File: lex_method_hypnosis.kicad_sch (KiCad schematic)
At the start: 4 parts

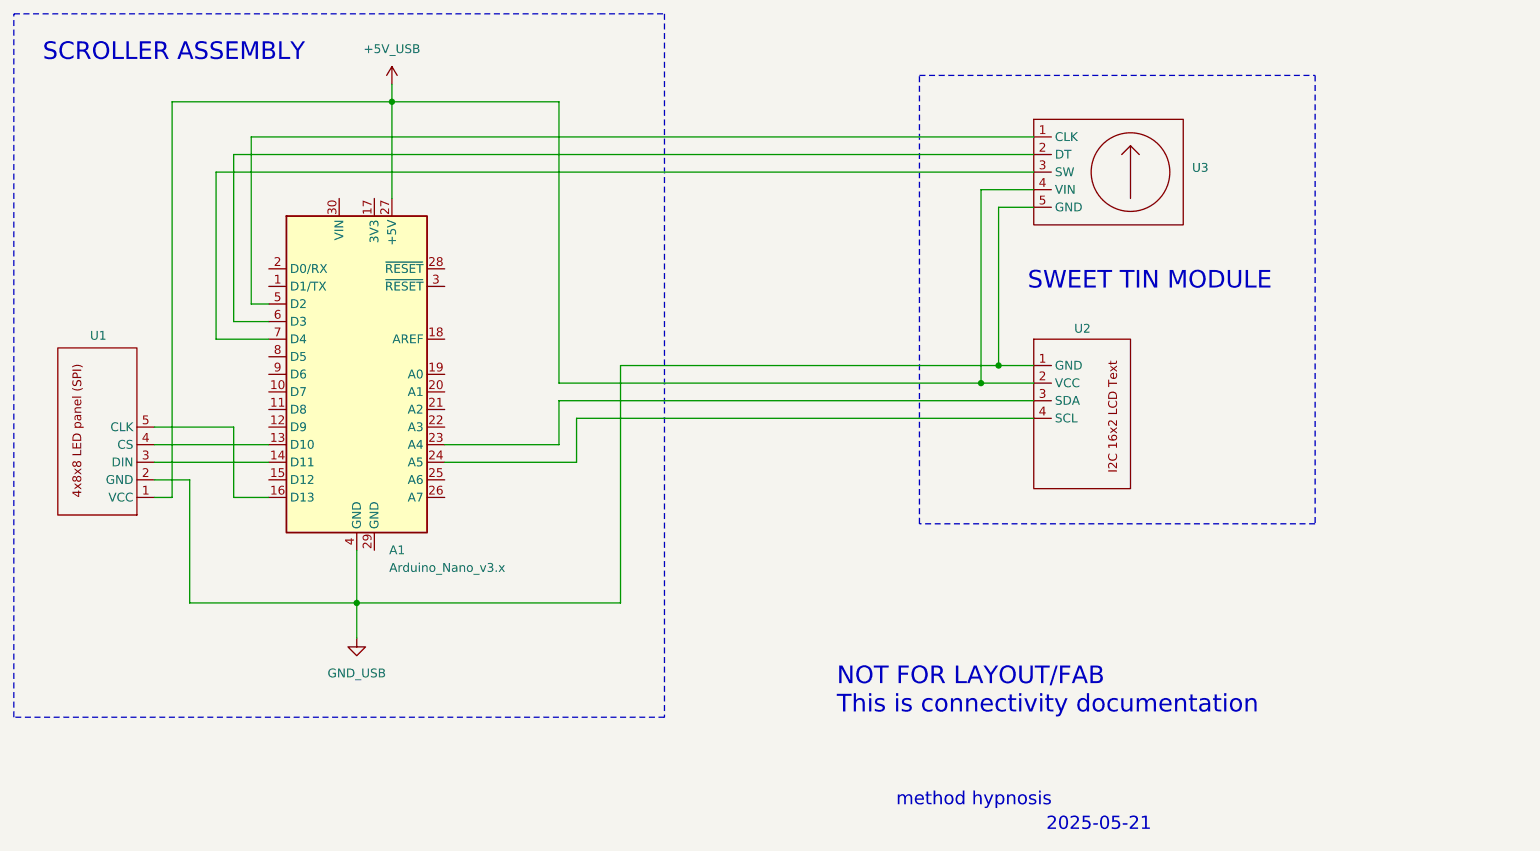
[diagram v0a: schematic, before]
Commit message: About to wire up connectors (gulpoid)
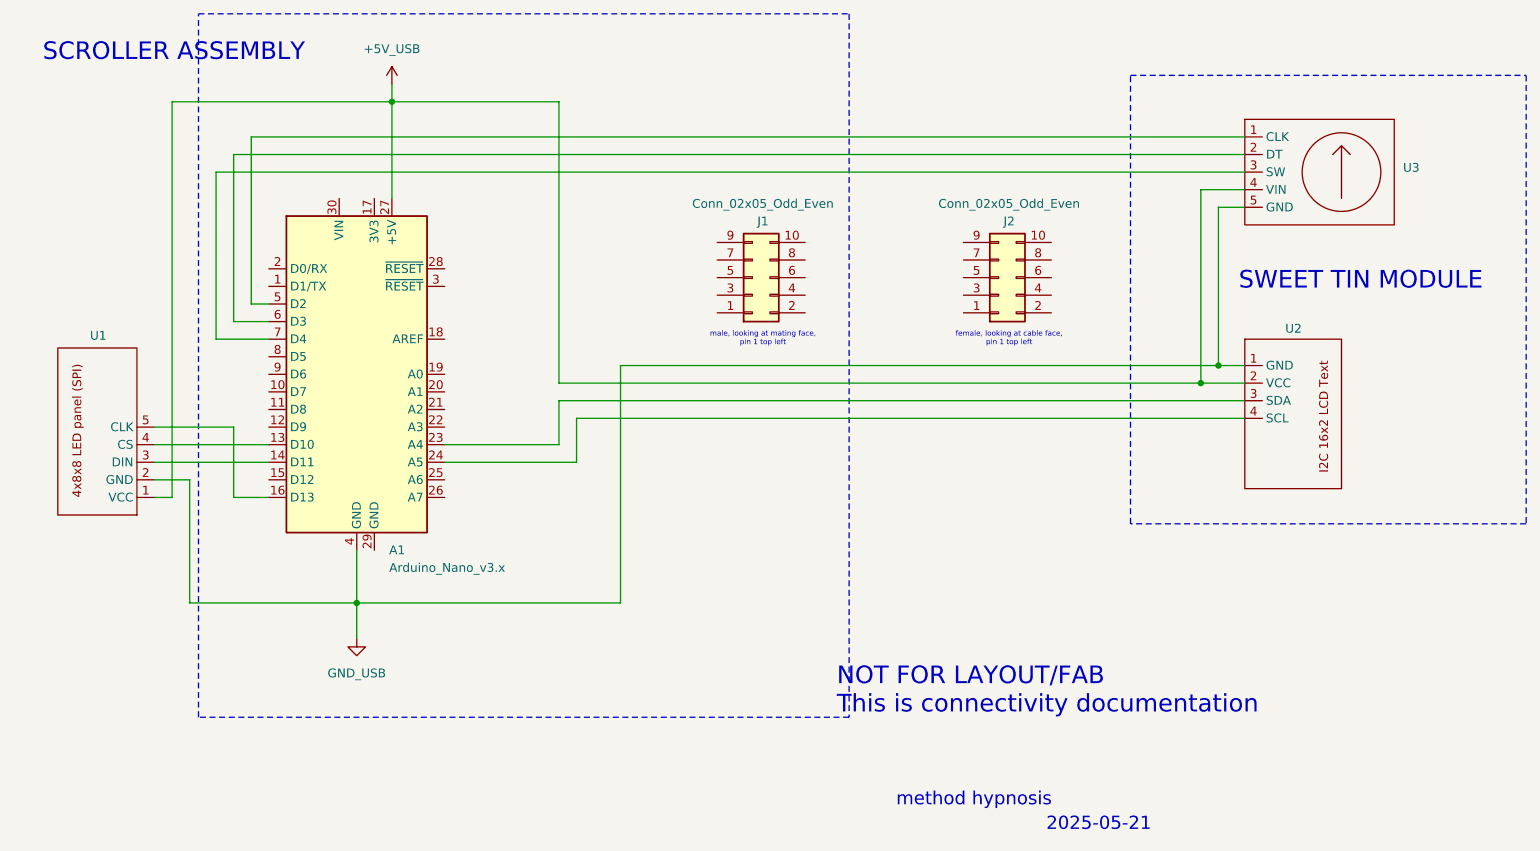
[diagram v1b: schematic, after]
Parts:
- added J1, J2: Conn_02x05_Odd_Even, symbol Connector_Generic:Conn_02x05_Odd_Even
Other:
- note added: "female, looking at cable face, pin 1 top left"
- note added: "male, looking at mating face, pin 1 top left"
- moved on the sheet: U2, U3
